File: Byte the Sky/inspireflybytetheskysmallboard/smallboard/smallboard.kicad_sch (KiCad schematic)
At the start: 15 parts, among them IC1 N34TS04MT3ETG, J1 Conn_01x07_Pin, U2 LSM6DSV, U4 LIS2MDLTR

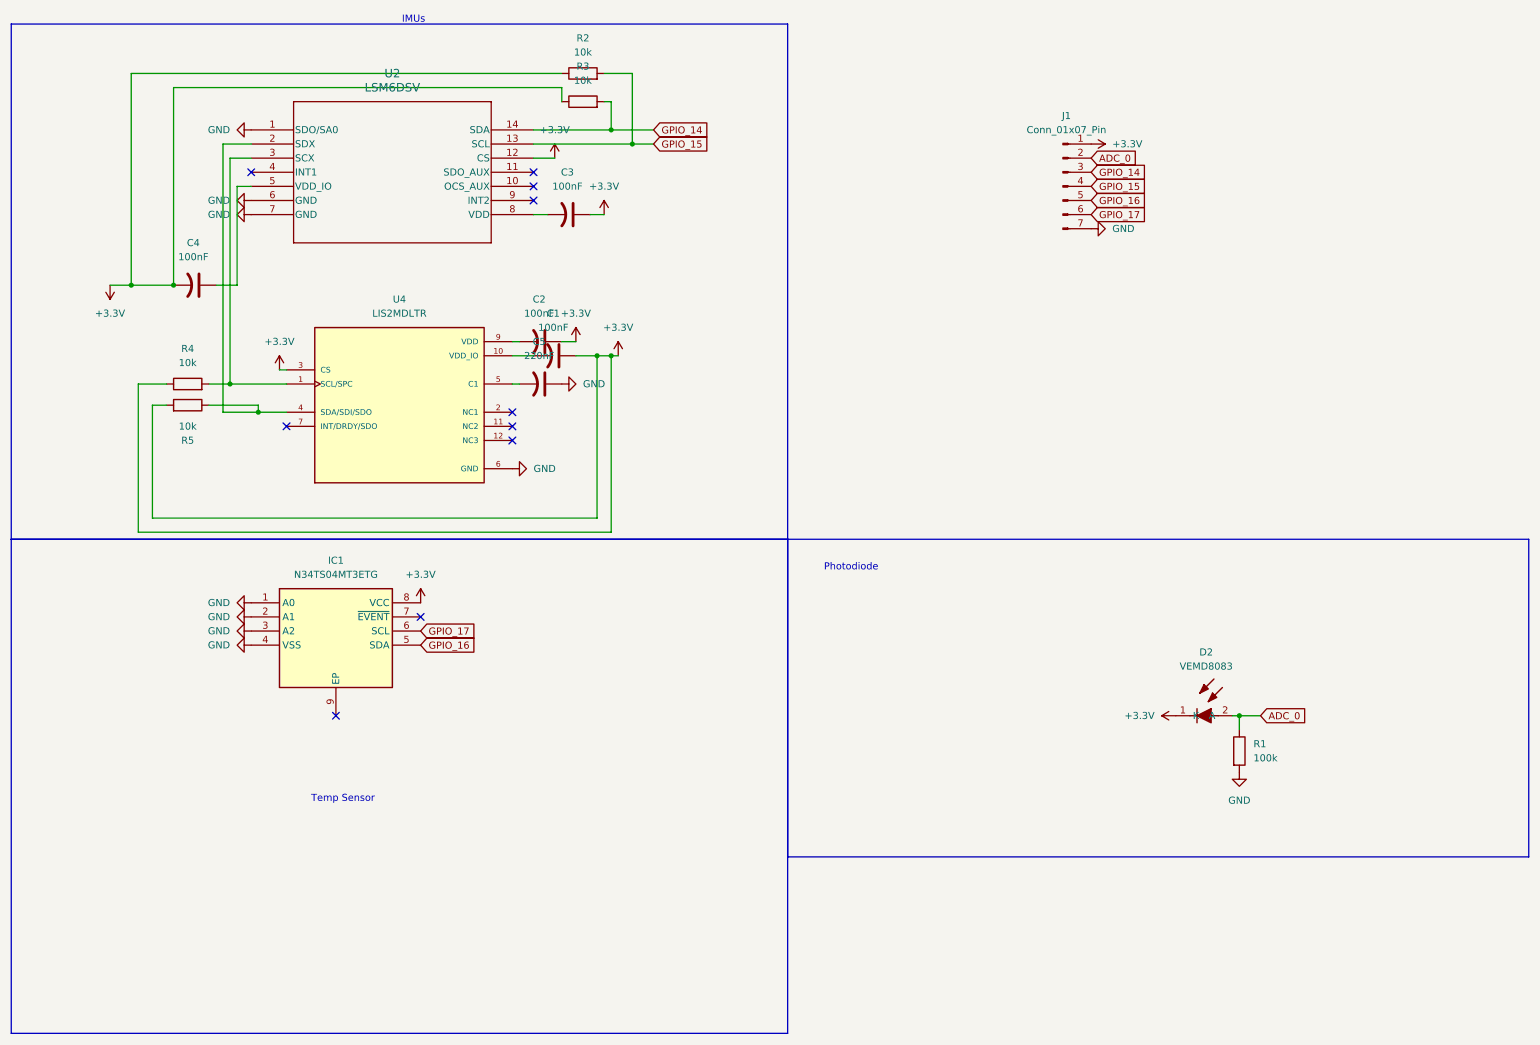
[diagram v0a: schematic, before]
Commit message: Add files via upload
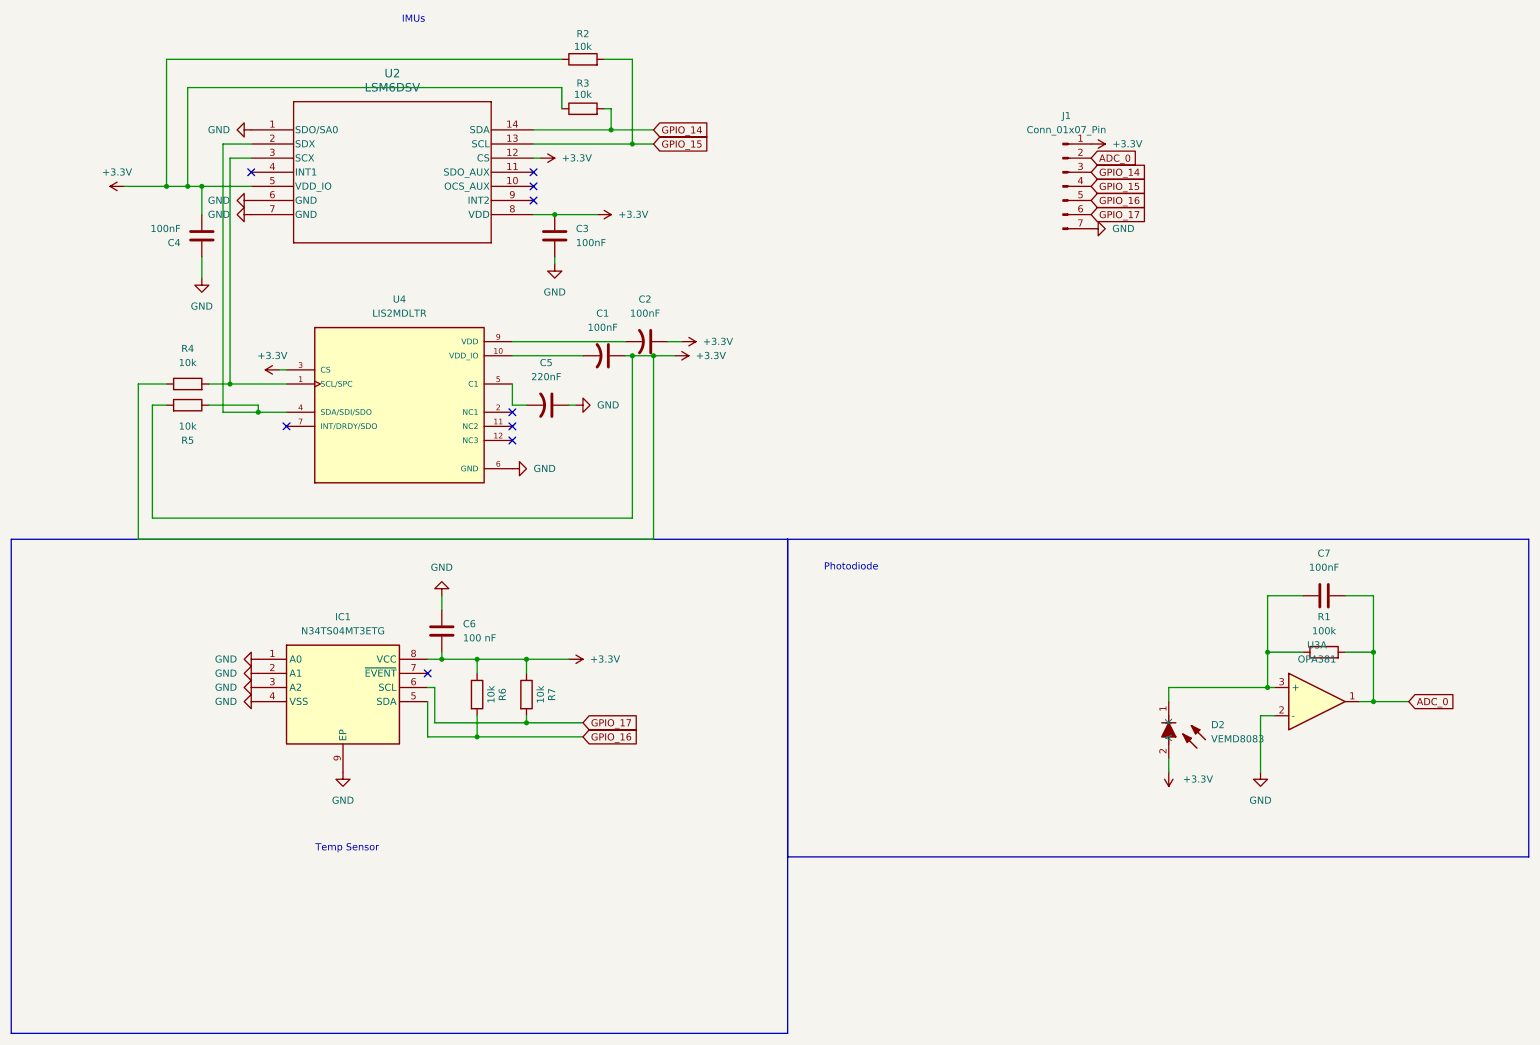
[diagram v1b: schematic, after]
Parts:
- removed C4: 100nF, Capacitor_SMD:C_0402_1005Metric, symbol Device:C_US
- added C4, C7: 100nF, Capacitor_SMD:C_0402_1005Metric, symbol Device:C
- added C6: 100 nF, Capacitor_SMD:C_0402_1005Metric, symbol Device:C
- added R6, R7: 10k, Resistor_SMD:R_0402_1005Metric, symbol Device:R
- added U3: OPA381, OPA381:MSOP08, symbol Device:Opamp_Dual
- C3: symbol Device:C_US -> Device:C
- D2: footprint VEMD:VEMD8083 -> footprints:VEMD8083
- IC1: footprint N34:SON50P300X200X80-9N -> footprints:SON50P300X200X80-9N
- U4: footprint LIS2MDLTR:PQFN50P200X200X70-12N -> footprints:PQFN50P200X200X70-12N
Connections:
- net +3.3V: now also D2.2 (A), U2.5 (VDD_IO), U2.8 (VDD), C4.2, C6.2, R6.1, R7.1; no longer D2.1 (K)
- net ADC_0: now also R1.2, C7.2, U3.1; no longer D2.2 (A), R1.1
- net GND: now also C3.2, IC1.9 (EP), C4.1, C6.1, U3.2 (-); no longer R1.2
- net GPIO_16: now also R6.2
- net GPIO_17: now also R7.2
- new net: C7.1, D2.1 (K), R1.1, U3.3 (+)
- no-connect marks 10 -> 9
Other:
- moved on the sheet: C1, C2, C3, C5, D2, IC1, R1, R2, R3
